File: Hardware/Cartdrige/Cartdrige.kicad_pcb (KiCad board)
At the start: 2 copper layers, 47.6 x 112.1 mm, 5 parts, among them J1 CARTDRIGE, U1 28C256, U2 28C256

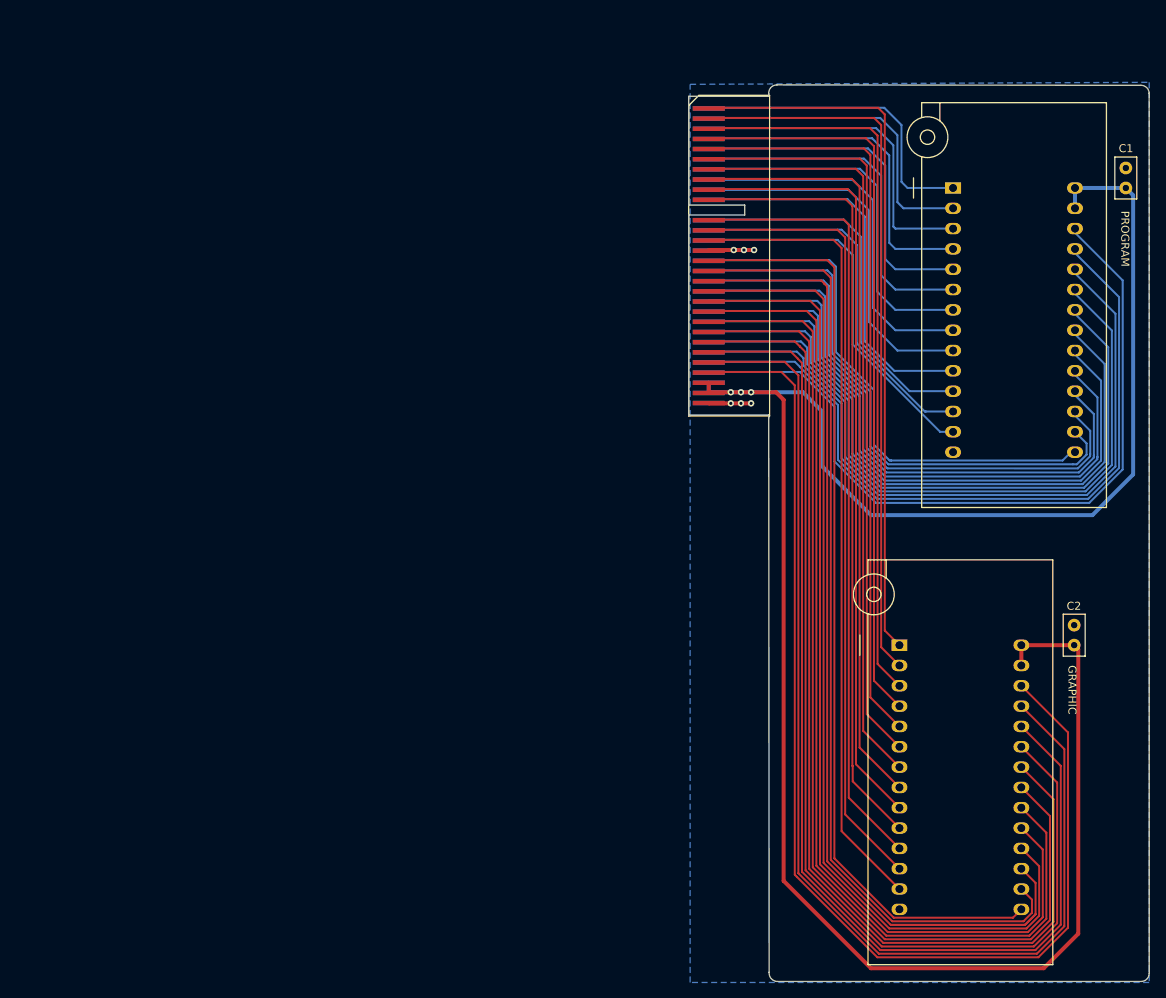
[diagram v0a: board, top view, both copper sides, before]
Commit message: Fix
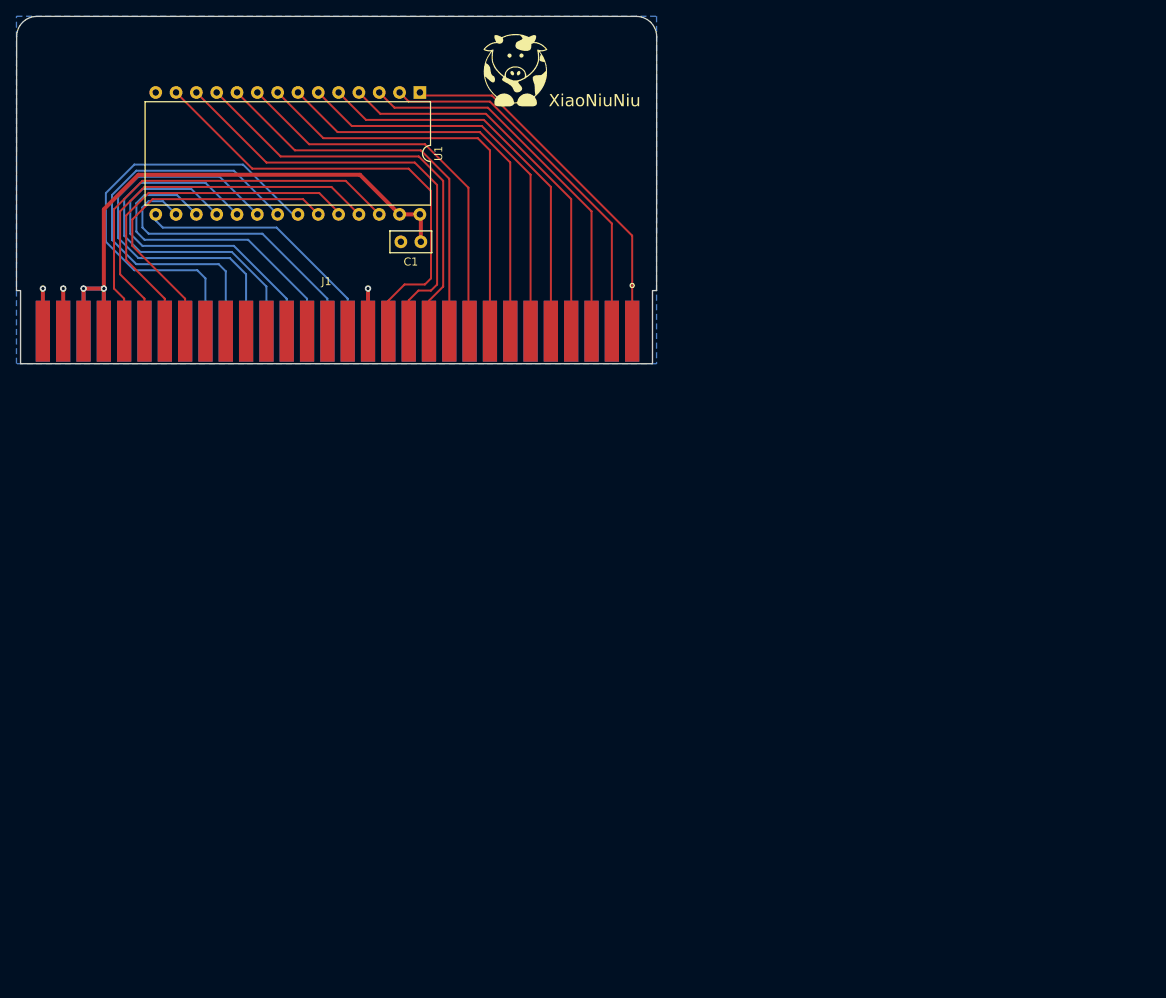
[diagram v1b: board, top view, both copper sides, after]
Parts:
- removed C2: 100nF, Capacitor_THT:C_Disc_D5.0mm_W2.5mm_P2.50mm
- removed U2: 28C256, Socket:DIP_Socket-28_W11.9_W12.7_W15.24_W17.78_W18.5_3M_228-1277-00-0602J
- added XiaoNiuNiu: LOGO, Logos:VerySmallCow, F.Cu at (87.9, 32.0)
- J1: value CARTDRIGE -> ROM; footprint Connector_PCBEdge:Samtec_MECF-30-0_-L-DV_2x30_P1.27mm_Polarized_Edge -> Connector_TheRLab:NES_PCBEdge
- U1: footprint Socket:DIP_Socket-28_W11.9_W12.7_W15.24_W17.78_W18.5_3M_228-1277-00-0602J -> Package_DIP:DIP-28_W15.24mm
- moved U1 91.5 mm to (75.9, 34.8), turned to -90 degrees
- moved C1 88.4 mm to (76.1, 53.5), turned to 180 degrees
- moved J1 51.1 mm to (64.4, 64.6), turned to 0 degrees
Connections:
- net /AA14 renamed /A14
- J1 pad 10: /AB5 -> /A0
- J1 pad 11: /AA4 -> /D0
- J1 pad 12: /AB4 -> /D1
- J1 pad 13: /AA3 -> /D2
- J1 pad 14: /AB3 -> GND
- J1 pad 15: /AA2 -> /D3
- J1 pad 16: /AB2 -> /D4
- J1 pad 17: /AA1 -> /D5
- J1 pad 18: /AB1 -> /D6
- J1 pad 19: /AA0 -> /D7
- J1 pad 2: /AB14 -> /A12
- J1 pad 20: /AB0 -> CS
- J1 pad 23: /DA0 -> /A11
- J1 pad 24: /DB0 -> /A9
- J1 pad 25: /DA1 -> /A8
- J1 pad 26: /DB1 -> /A13
- J1 pad 27: /DA2 -> +5V
- J1 pad 28: /DB2 -> +5V
- J1 pad 3: /AA12 -> /A7
- J1 pad 4: /AB12 -> /A6
- J1 pad 5: /AA7 -> /A5
- J1 pad 6: /AB7 -> /A4
- J1 pad 7: /AA6 -> /A3
- J1 pad 8: /AB6 -> /A2
- J1 pad 9: /AA5 -> /A1
- U1 pad 10: /AA0 -> /A0
- U1 pad 11: /DA0 -> /D0
- U1 pad 12: /DA1 -> /D1
- U1 pad 13: /DA2 -> /D2
- U1 pad 15: /DA3 -> /D3
- U1 pad 16: /DA4 -> /D4
- U1 pad 17: /DA5 -> /D5
- U1 pad 18: /DA6 -> /D6
- U1 pad 19: /DA7 -> /D7
- U1 pad 2: /AA12 -> /A12
- U1 pad 20: CSA -> CS
- U1 pad 21: /AA10 -> /A10
- U1 pad 22: OEA -> OE
- U1 pad 23: /AA11 -> /A11
- U1 pad 24: /AA9 -> /A9
- U1 pad 25: /AA8 -> /A8
- U1 pad 26: /AA13 -> /A13
- U1 pad 3: /AA7 -> /A7
- U1 pad 4: /AA6 -> /A6
- U1 pad 5: /AA5 -> /A5
- U1 pad 6: /AA4 -> /A4
- U1 pad 7: /AA3 -> /A3
- U1 pad 8: /AA2 -> /A2
- U1 pad 9: /AA1 -> /A1
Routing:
- net +5V: track 271.5 -> 83.3 mm, vias 3 -> 2
- net /AA13: track 145.2 -> 0.00 mm
- net /AA8: track 142.7 -> 0.00 mm
- net /DA5: track 141.9 -> 0.00 mm
- net /AA9: track 140.4 -> 0.00 mm
- net /AA11: track 137.9 -> 0.00 mm
- net OEA: track 135.5 -> 0.00 mm
- net /AA10: track 133.0 -> 0.00 mm
- net CSA: track 130.5 -> 0.00 mm
- net /DA7: track 128.0 -> 0.00 mm
- net /DA6: track 125.6 -> 0.00 mm
- net /DA4: track 120.7 -> 0.00 mm
- net /DA3: track 116.8 -> 0.00 mm
- net /DA2: track 100.1 -> 0.00 mm
- net /DA1: track 99.2 -> 0.00 mm
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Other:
- board size 47.6 x 112.1 mm -> 80 x 34.3 mm
- board text removed: "GRAPHIC"
- board text removed: "PROGRAM"
